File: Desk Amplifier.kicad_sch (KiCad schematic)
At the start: 37 parts, among them J1 STX-3000, J2 STX-3000, J3 STX-3000, J4 STX-3000, J6 USB4970-00-A, U1 OPA2134, U2 OPA2134

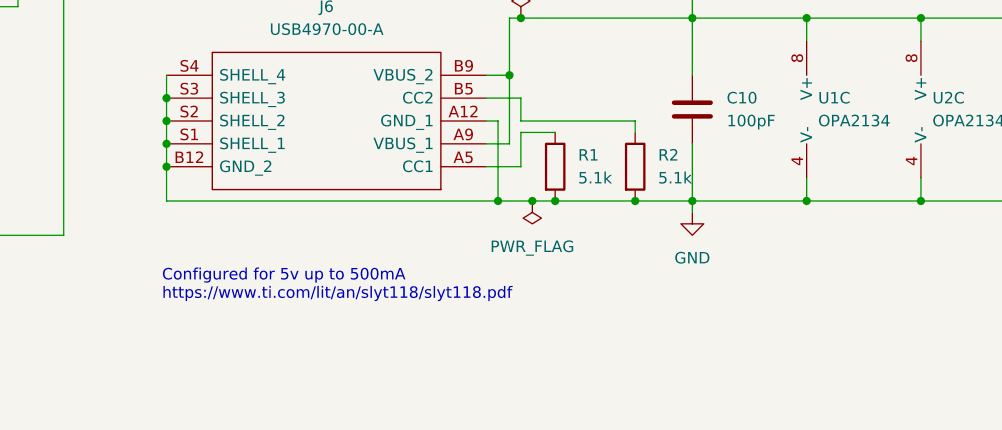
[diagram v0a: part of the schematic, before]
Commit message: fixup routing
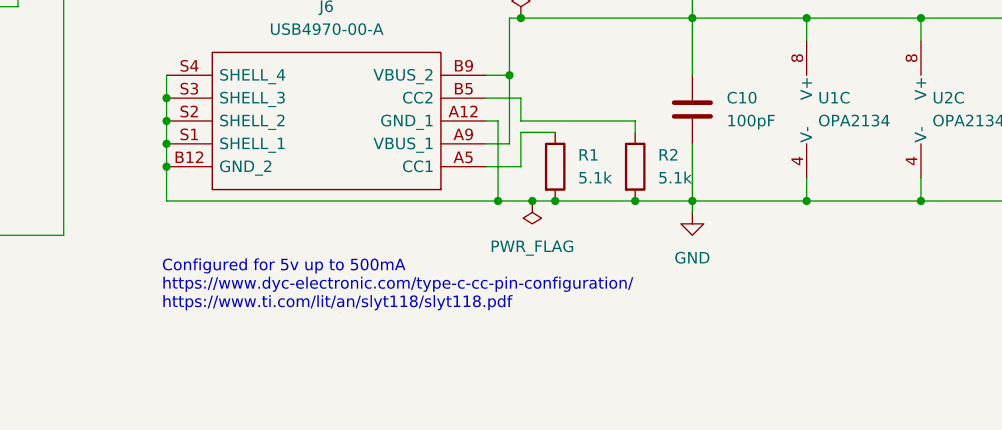
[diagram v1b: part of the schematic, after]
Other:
- note added: "Configured for 5v up to 500mA https://www.dyc-electronic.com/type-c-cc-pin-configuration/ https://www.ti.com/lit/an/slyt118/slyt118.pdf"
- note removed: "Configured for 5v up to 500mA https://www.ti.com/lit/an/slyt118/slyt118.pdf"
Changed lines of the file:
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@@
 		)
 	)
-	(text "Configured for 5v up to 500mA\nhttps://www.ti.com/lit/an/slyt118/slyt118.pdf"
+	(text "Configured for 5v up to 500mA\nhttps://www.dyc-electronic.com/type-c-cc-pin-configuration/\nhttps://www.ti.com/lit/an/slyt118/slyt118.pdf"
 		(exclude_from_sim no)
 		(at 126.492 150.368 0)

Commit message: fix nets & round corners
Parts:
- H1, H2, H3: footprint MountingHole:MountingHole_2.1mm -> MountingHole:MountingHole_2.5mm
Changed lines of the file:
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@@
 			)
 		)
-		(property "Footprint" "MountingHole:MountingHole_2.1mm"
+		(property "Footprint" "MountingHole:MountingHole_2.5mm"
 			(at 262.89 99.06 0)
 			(hide yes)
@@
 			)
 		)
-		(property "Footprint" "MountingHole:MountingHole_2.1mm"
+		(property "Footprint" "MountingHole:MountingHole_2.5mm"
 			(at 262.89 109.22 0)
 			(hide yes)
@@
 			)
 		)
-		(property "Footprint" "MountingHole:MountingHole_2.1mm"
+		(property "Footprint" "MountingHole:MountingHole_2.5mm"
 			(at 262.89 104.14 0)
 			(hide yes)
